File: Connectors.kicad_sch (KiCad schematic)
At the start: 10 parts, among them J10 200528-0100, J11 200528-0100, J12 200528-0100, J13 282834-6, J18 200528-0100, J5 200528-0100, J6 200528-0100, J7 200528-0100, J8 200528-0100, J9 200528-0100

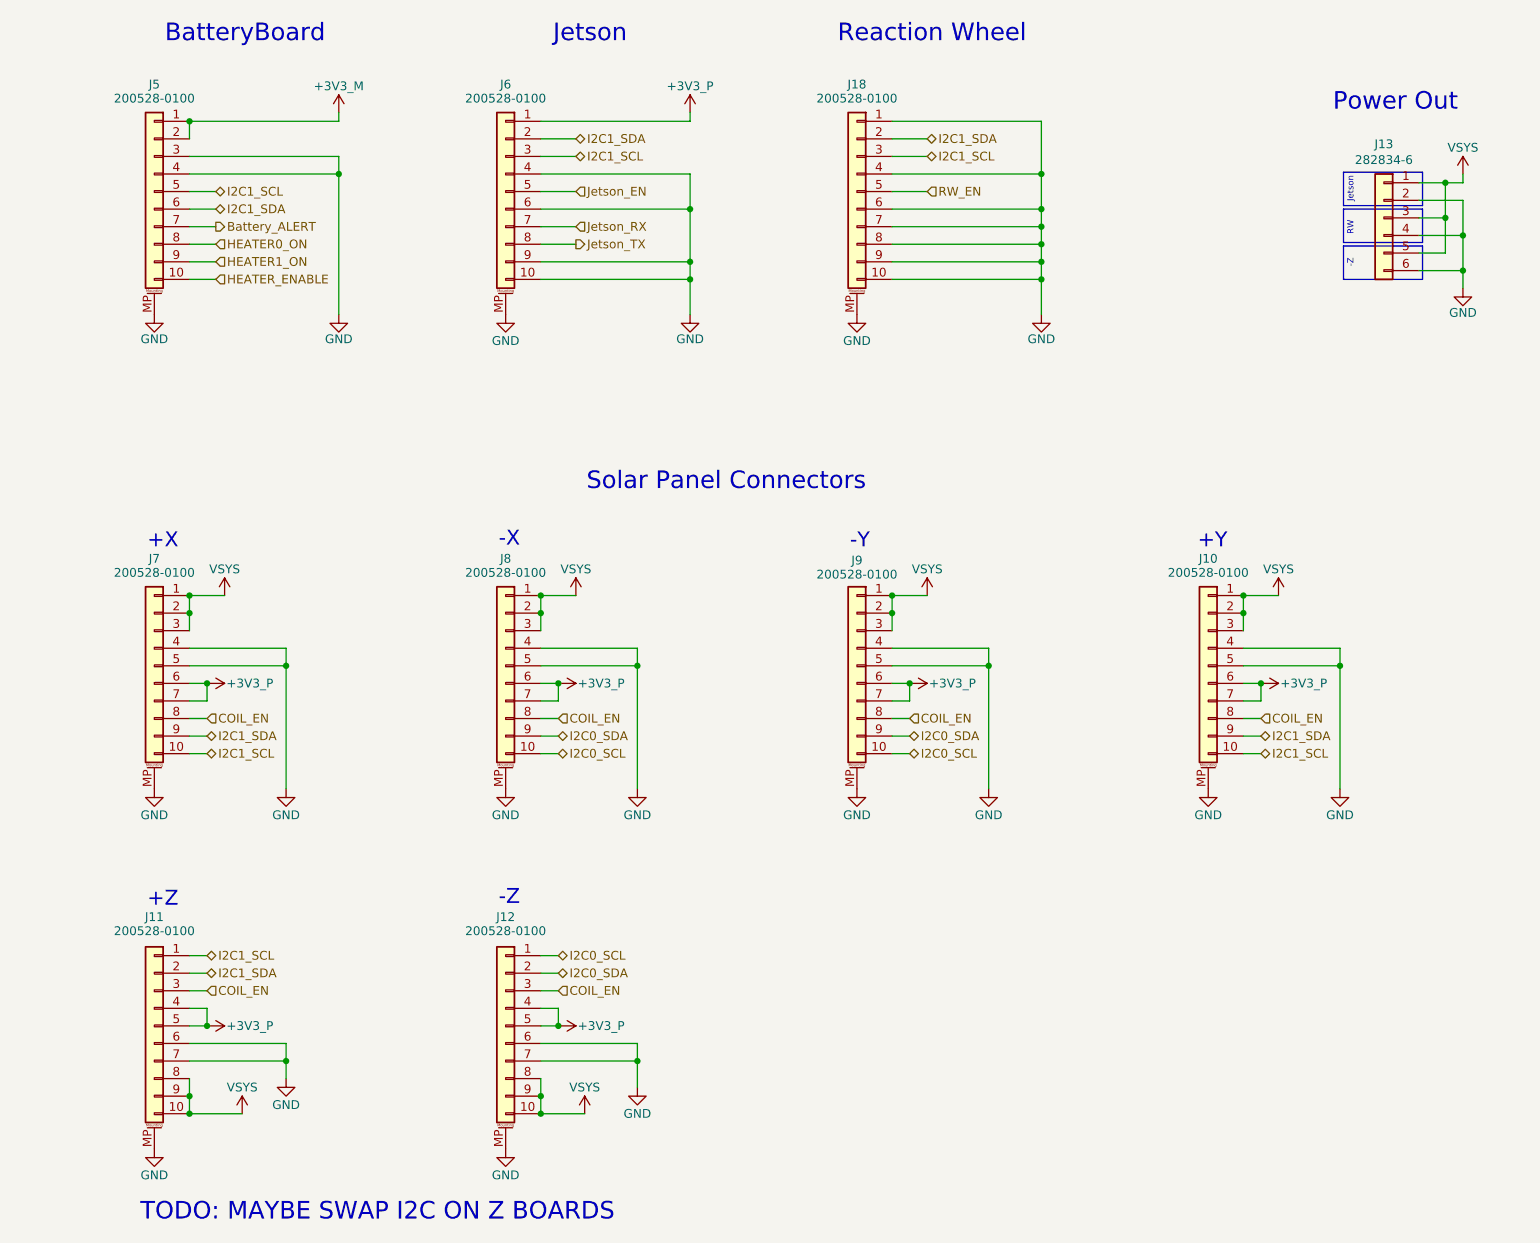
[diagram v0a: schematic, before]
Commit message: v4.0 Updates
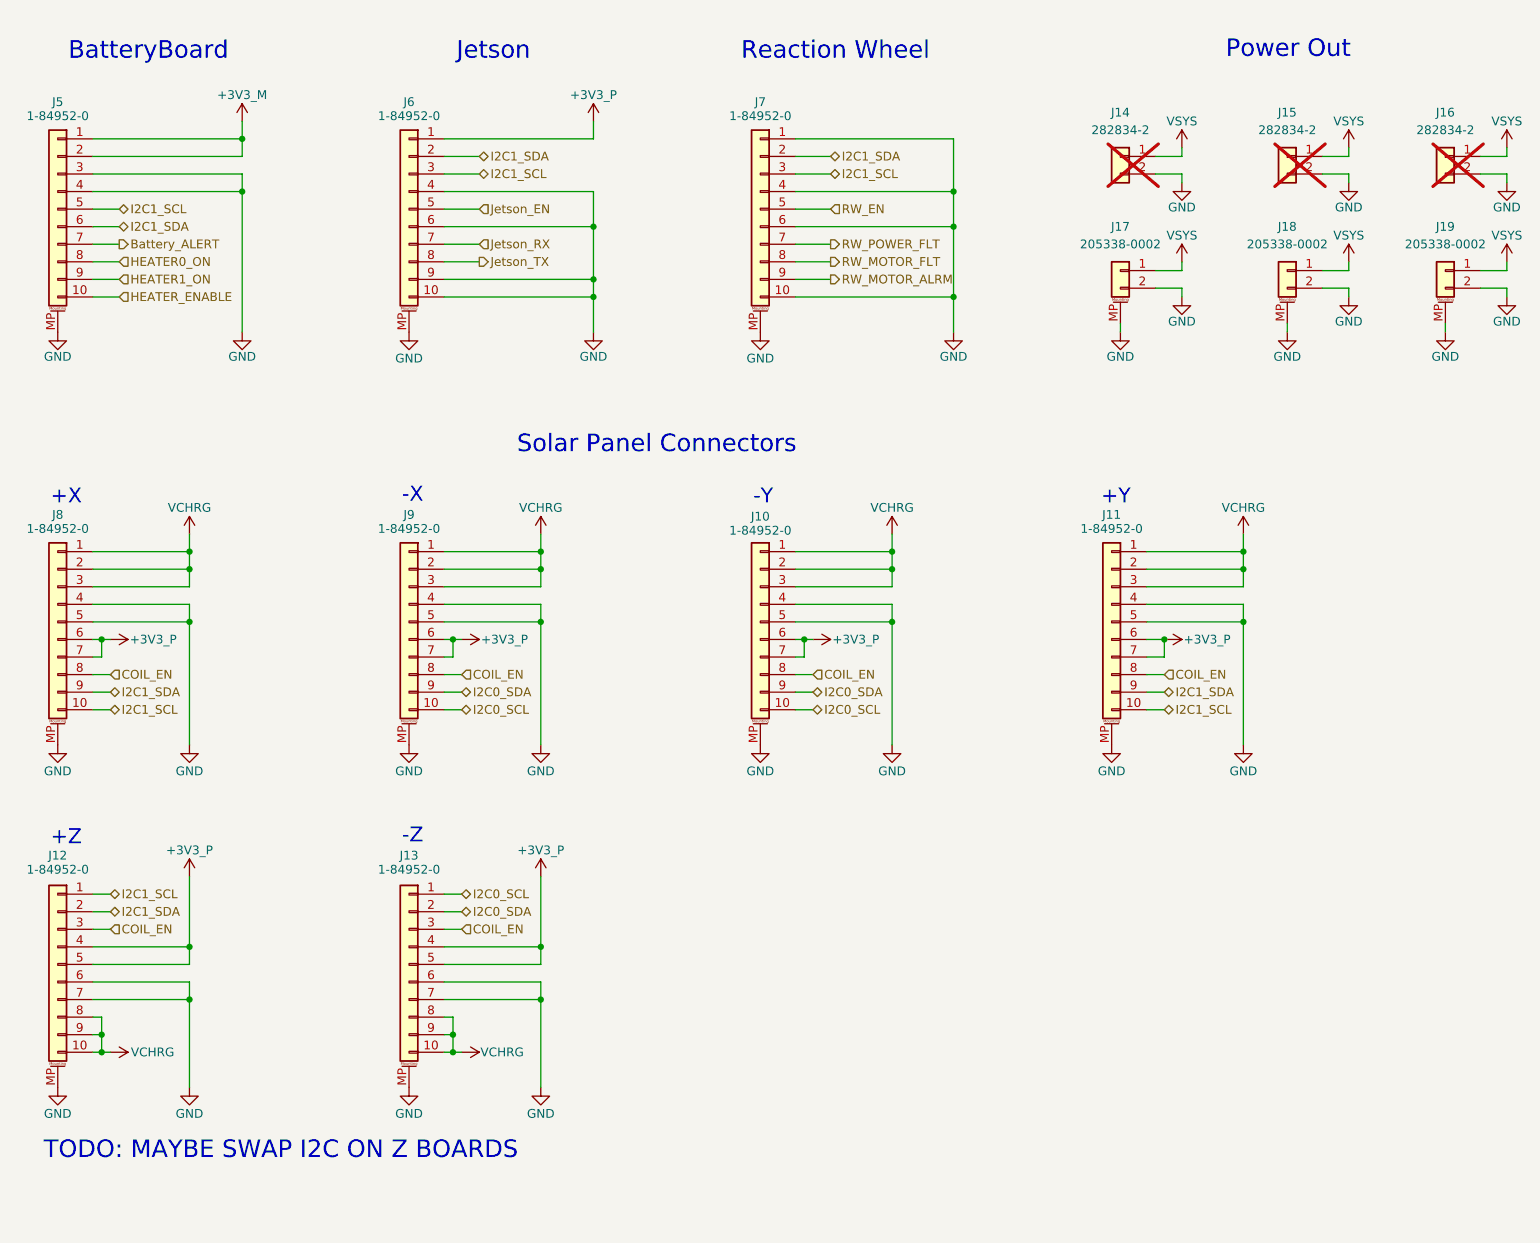
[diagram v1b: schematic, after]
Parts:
- removed J13: 282834-6, Argus-Connectors:TE_282834-6, symbol Connector_Generic:Conn_01x06
- added J14, J15, J16: 282834-2, Argus-Connectors:TE_282834-2, symbol Connector_Generic:Conn_01x02
- added J17, J18, J19: 205338-0002, Connector_Molex:Molex_Pico-Lock_205338-0002_1x02-1MP_P2.00mm_Horizontal, symbol Connector_Generic_MountingPin:Conn_01x02_MountingPin
- J10: renamed from J9; value 200528-0100 -> 1-84952-0; footprint Argus-Connectors:Molex_200528-0100_1x10-1MP_P1.00mm_Horizontal -> Argus-Connectors:CON_522711069_MOL
- J11: renamed from J10; value 200528-0100 -> 1-84952-0; footprint Argus-Connectors:Molex_200528-0100_1x10-1MP_P1.00mm_Horizontal -> Argus-Connectors:CON_522711069_MOL
- J12: renamed from J11; value 200528-0100 -> 1-84952-0; footprint Argus-Connectors:Molex_200528-0100_1x10-1MP_P1.00mm_Horizontal -> Argus-Connectors:CON_522711069_MOL
- J13: renamed from J12; value 200528-0100 -> 1-84952-0; footprint Argus-Connectors:Molex_200528-0100_1x10-1MP_P1.00mm_Horizontal -> Argus-Connectors:CON_522711069_MOL
- J5, J6: value 200528-0100 -> 1-84952-0; footprint Argus-Connectors:Molex_200528-0100_1x10-1MP_P1.00mm_Horizontal -> Argus-Connectors:CON_522711069_MOL
- J7: renamed from J18; value 200528-0100 -> 1-84952-0; footprint Argus-Connectors:Molex_200528-0100_1x10-1MP_P1.00mm_Horizontal -> Argus-Connectors:CON_522711069_MOL
- J8: renamed from J7; value 200528-0100 -> 1-84952-0; footprint Argus-Connectors:Molex_200528-0100_1x10-1MP_P1.00mm_Horizontal -> Argus-Connectors:CON_522711069_MOL
- J9: renamed from J8; value 200528-0100 -> 1-84952-0; footprint Argus-Connectors:Molex_200528-0100_1x10-1MP_P1.00mm_Horizontal -> Argus-Connectors:CON_522711069_MOL
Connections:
- net GND: now also J14.2 (Pin_2), J15.2 (Pin_2), J16.2 (Pin_2), J17.2 (Pin_2), J17.MP (MountPin), J18.2 (Pin_2), J18.MP (MountPin), J19.2 (Pin_2), J19.MP (MountPin); no longer J7.7 (Pin_7), J7.8 (Pin_8), J7.9 (Pin_9)
- net VSYS: now also J14.1 (Pin_1), J15.1 (Pin_1), J16.1 (Pin_1), J17.1 (Pin_1), J18.1 (Pin_1), J19.1 (Pin_1); no longer J10.1 (Pin_1), J10.2 (Pin_2), J10.3 (Pin_3), J11.1 (Pin_1), J11.2 (Pin_2), J11.3 (Pin_3), J12.10 (Pin_10), J12.8 (Pin_8), J12.9 (Pin_9), J13.10 (Pin_10), J13.8 (Pin_8), J13.9 (Pin_9), J8.1 (Pin_1), J8.2 (Pin_2), J8.3 (Pin_3), J9.1 (Pin_1), J9.2 (Pin_2), J9.3 (Pin_3)
- new net RW_MOTOR_ALRM: J7.9 (Pin_9)
- new net RW_MOTOR_FLT: J7.8 (Pin_8)
- new net RW_POWER_FLT: J7.7 (Pin_7)
- new net VCHRG: J10.1 (Pin_1), J10.2 (Pin_2), J10.3 (Pin_3), J11.1 (Pin_1), J11.2 (Pin_2), J11.3 (Pin_3), J12.10 (Pin_10), J12.8 (Pin_8), J12.9 (Pin_9), J13.10 (Pin_10), J13.8 (Pin_8), J13.9 (Pin_9), J8.1 (Pin_1), J8.2 (Pin_2), J8.3 (Pin_3), J9.1 (Pin_1), J9.2 (Pin_2), J9.3 (Pin_3)
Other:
- note removed: "RW"
- moved on the sheet: J10, J11, J12, J13, J5, J6, J7, J8, J9
